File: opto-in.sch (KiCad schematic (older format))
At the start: 4 parts, among them U5 4N25

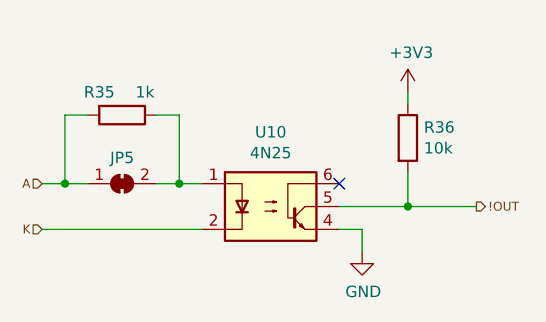
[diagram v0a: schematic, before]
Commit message: Several changes
Usando stock de http://tienda.ityt.com.ar/
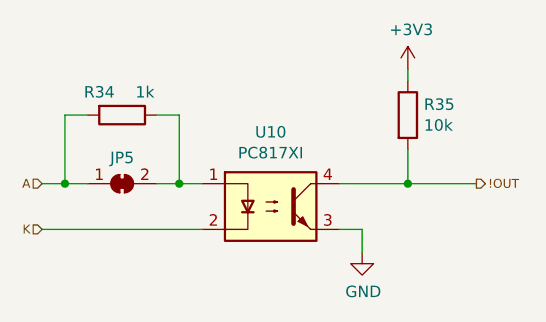
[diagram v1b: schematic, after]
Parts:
- removed U5: 4N25, Package_DIP:DIP-6_W7.62mm, symbol Isolator:4N25
- added U5: PC817XI, Package_DIP:SMDIP-4_W9.53mm, symbol Isolator:PC817
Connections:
- net !OUT: now also U5.4
- net GND: now also U5.3
- net K: now also U5.2
- net at JP3.2 (B), R31.1: now also U5.1
- no-connect marks 1 -> 0
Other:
- moved on the sheet: R35
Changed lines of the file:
@@
 $Descr A4 11693 8268
 encoding utf-8
-Sheet 17 19
+Sheet 16 18
 Title "Opto-coupled Input"
 Date "2021-06-10"
@@
 $EndDescr
 $Comp
-L Isolator:4N25 U?
-U 1 1 6144C515
-P 5550 4050
-AR Path="/6144C515" Ref="U?"  Part="1"
-AR Path="/61400494/61448E8E/6144C515" Ref="U?"  Part="1"
-AR Path="/61400494/614555D4/6144C515" Ref="U5"  Part="1"
-AR Path="/61400494/61466DF4/6144C515" Ref="U8"  Part="1"
-AR Path="/61400494/61467145/6144C515" Ref="U10"  Part="1"
-F 0 "U10" H 5550 4375 50  0000 C CNN
-F 1 "4N25" H 5550 4284 50  0000 C CNN
-F 2 "Package_DIP:DIP-6_W7.62mm" H 5350 3850 50  0001 L CIN
-F 3 "https://optoelectronics.liteon.com/upload/download/DS-70-99-0010/4N2X%20series%20Datasheet%201115.pdf" H 5550 4050 50  0001 L CNN
-F 4 "4N25" H 5550 4050 50  0001 C CNN "manf#"
-	1    5550 4050
-	1    0    0    -1
-$EndComp
-$Comp
 L power:+3V3 #PWR?
 U 1 1 6144C538
-P 6150 3550
+P 6150 3450
 AR Path="/6144C538" Ref="#PWR?"  Part="1"
 AR Path="/61400494/61448E8E/6144C538" Ref="#PWR?"  Part="1"
@@
 AR Path="/61400494/61466DF4/6144C538" Ref="#PWR0153"  Part="1"
 AR Path="/61400494/61467145/6144C538" Ref="#PWR0155"  Part="1"
-F 0 "#PWR0155" H 6150 3400 50  0001 C CNN
-F 1 "+3V3" H 6165 3723 50  0000 C CNN
-F 2 "" H 6150 3550 50  0001 C CNN
-F 3 "" H 6150 3550 50  0001 C CNN
-	1    6150 3550
+AR Path="/60DA21D5/6144C538" Ref="#PWR0148"  Part="1"
+AR Path="/60DA21DD/6144C538" Ref="#PWR0150"  Part="1"
+AR Path="/60DA21E2/6144C538" Ref="#PWR0152"  Part="1"
+F 0 "#PWR0152" H 6150 3300 50  0001 C CNN
+F 1 "+3V3" H 6165 3623 50  0000 C CNN
+F 2 "" H 6150 3450 50  0001 C CNN
+F 3 "" H 6150 3450 50  0001 C CNN
+	1    6150 3450
 	1    0    0    -1
 $EndComp
 Wire Wire Line
-	6150 3600 6150 3550
-Text HLabel 6450 4050 2    39   Output ~ 0
+	6150 3500 6150 3450
+Text HLabel 6450 3950 2    39   Output ~ 0
 !OUT
 Text HLabel 4550 3950 0    39   Input ~ 0
@@
 AR Path="/61400494/61466DF4/6145BF52" Ref="#PWR0154"  Part="1"
 AR Path="/61400494/61467145/6145BF52" Ref="#PWR0156"  Part="1"
-F 0 "#PWR0156" H 5950 4000 50  0001 C CNN
+AR Path="/60DA21D5/6145BF52" Ref="#PWR0149"  Part="1"
+AR Path="/60DA21DD/6145BF52" Ref="#PWR0151"  Part="1"
+AR Path="/60DA21E2/6145BF52" Ref="#PWR0153"  Part="1"
+F 0 "#PWR0153" H 5950 4000 50  0001 C CNN
 F 1 "GND" H 5955 4077 50  0000 C CNN
 F 2 "" H 5950 4250 50  0001 C CNN
@@
 L Device:R R32
 U 1 1 6145DEBF
-P 6150 3750
+P 6150 3650
 AR Path="/61400494/614555D4/6145DEBF" Ref="R32"  Part="1"
 AR Path="/61400494/61466DF4/6145DEBF" Ref="R34"  Part="1"
 AR Path="/61400494/61467145/6145DEBF" Ref="R36"  Part="1"
-F 0 "R36" H 6220 3796 50  0000 L CNN
-F 1 "10k" H 6220 3705 50  0000 L CNN
-F 2 "Resistor_SMD:R_1206_3216Metric" V 6080 3750 50  0001 C CNN
-F 3 "https://www.yageo.com/upload/media/product/productsearch/datasheet/rchip/PYu-RC_Group_51_RoHS_L_11.pdf" H 6150 3750 50  0001 C CNN
-F 4 "RC1206FR-0710KL" H 6150 3750 50  0001 C CNN "manf#"
-	1    6150 3750
+AR Path="/60DA21D5/6145DEBF" Ref="R31"  Part="1"
+AR Path="/60DA21DD/6145DEBF" Ref="R33"  Part="1"
+AR Path="/60DA21E2/6145DEBF" Ref="R35"  Part="1"
+F 0 "R35" H 6220 3696 50  0000 L CNN
+F 1 "10k" H 6220 3605 50  0000 L CNN
+F 2 "Resistor_SMD:R_1206_3216Metric" V 6080 3650 50  0001 C CNN
+F 3 "https://www.yageo.com/upload/media/product/productsearch/datasheet/rchip/PYu-RC_Group_51_RoHS_L_11.pdf" H 6150 3650 50  0001 C CNN
+F 4 "RC1206FR-0710KL" H 6150 3650 50  0001 C CNN "manf#"
+	1    6150 3650
 	1    0    0    -1
 $EndComp
 Wire Wire Line
-	5850 4050 6150 4050
+	5850 3950 6150 3950
 Wire Wire Line
-	6150 4050 6150 3900
+	6150 3950 6150 3800
 Wire Wire Line
-	6150 4050 6450 4050
-Connection ~ 6150 4050
-NoConn ~ 5850 3950
+	6150 3950 6450 3950
+Connection ~ 6150 3950
 $Comp
 L Device:R R31
@@
 AR Path="/61400494/61466DF4/61462D44" Ref="R33"  Part="1"
 AR Path="/61400494/61467145/61462D44" Ref="R35"  Part="1"
-F 0 "R35" V 4800 3550 50  0000 C CNN
+AR Path="/60DA21D5/61462D44" Ref="R30"  Part="1"
+AR Path="/60DA21DD/61462D44" Ref="R32"  Part="1"
+AR Path="/60DA21E2/61462D44" Ref="R34"  Part="1"
+F 0 "R34" V 4800 3550 50  0000 C CNN
 F 1 "1k" V 4800 3750 50  0000 C CNN
 F 2 "Resistor_SMD:R_1206_3216Metric" V 4830 3650 50  0001 C CNN
@@
 AR Path="/61400494/61466DF4/61464300" Ref="JP4"  Part="1"
 AR Path="/61400494/61467145/61464300" Ref="JP5"  Part="1"
+AR Path="/60DA21D5/61464300" Ref="JP3"  Part="1"
+AR Path="/60DA21DD/61464300" Ref="JP4"  Part="1"
+AR Path="/60DA21E2/61464300" Ref="JP5"  Part="1"
 F 0 "JP5" H 4900 4063 50  0000 C CNN
 F 1 "SolderJumper_2_Bridged" H 4900 4064 50  0001 C CNN
@@
 Wire Wire Line
 	4550 4150 5250 4150
+$Comp
+L Isolator:PC817 U?
+U 1 1 60DC8627
+P 5550 4050
+AR Path="/60DA21CE/60DC8627" Ref="U?"  Part="1"
+AR Path="/60DA21D5/60DC8627" Ref="U5"  Part="1"
+AR Path="/60DA21DD/60DC8627" Ref="U8"  Part="1"
+AR Path="/60DA21E2/60DC8627" Ref="U10"  Part="1"
+F 0 "U10" H 5550 4375 50  0000 C CNN
+F 1 "PC817XI" H 5550 4284 50  0000 C CNN
+F 2 "Package_DIP:SMDIP-4_W9.53mm" H 5350 3850 50  0001 L CIN
+F 3 "https://www.farnell.com/datasheets/73758.pdf" H 5550 4050 50  0001 L CNN
+F 4 "PC817XI" H 5550 4050 50  0001 C CNN "manf#"
+	1    5550 4050
+	1    0    0    -1
+$EndComp
 $EndSCHEMATC
